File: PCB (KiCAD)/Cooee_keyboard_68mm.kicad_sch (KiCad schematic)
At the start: 99 parts, among them J1 Conn_01x15_Pin

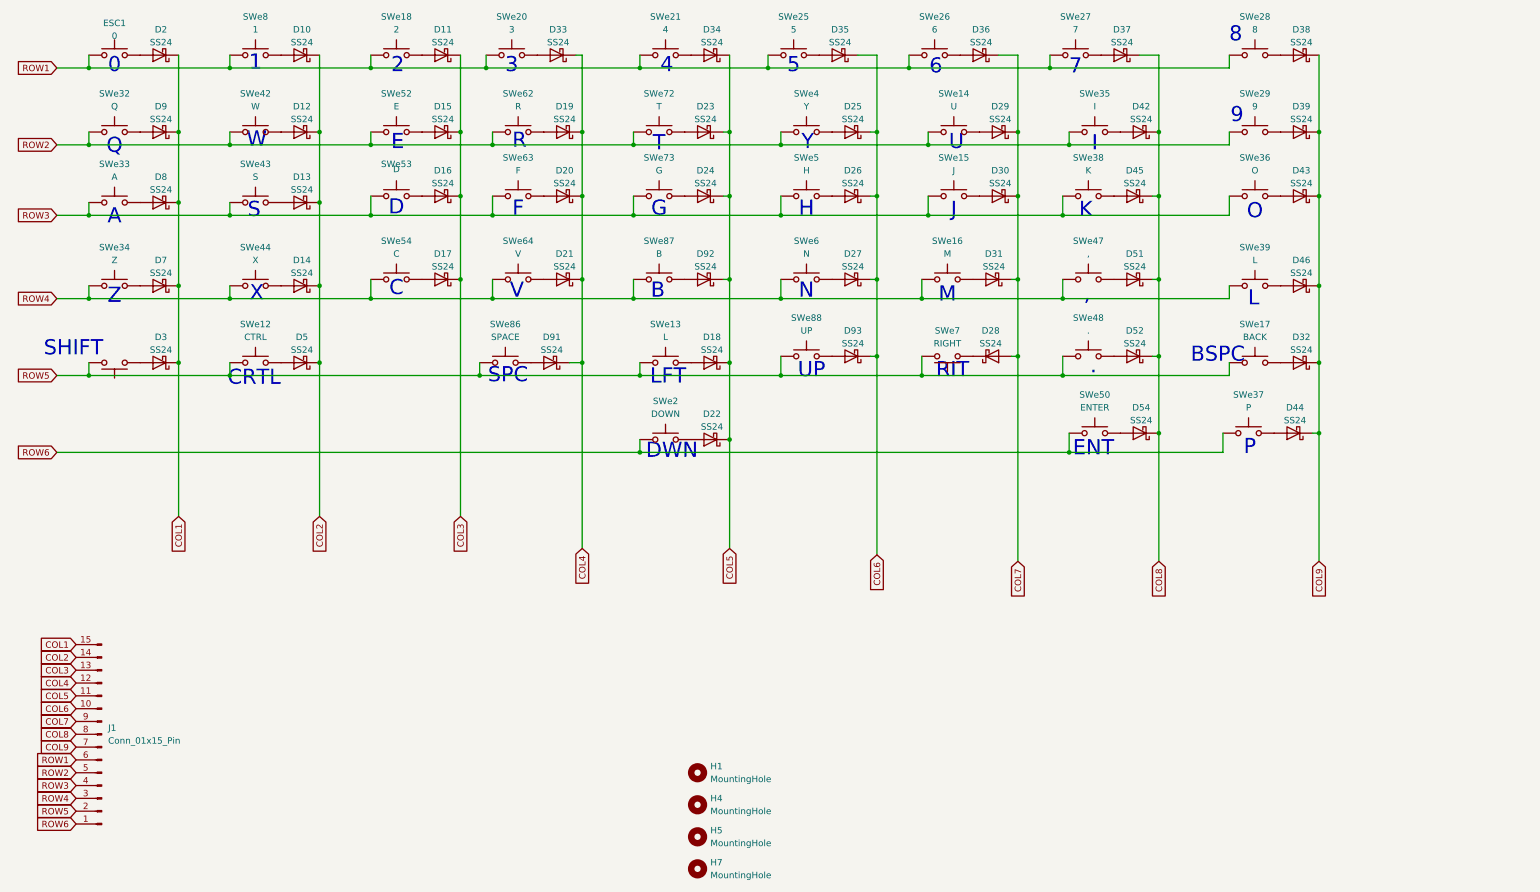
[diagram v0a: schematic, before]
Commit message: finished routing new smaller keyboard
finished routing new smaller keyboard
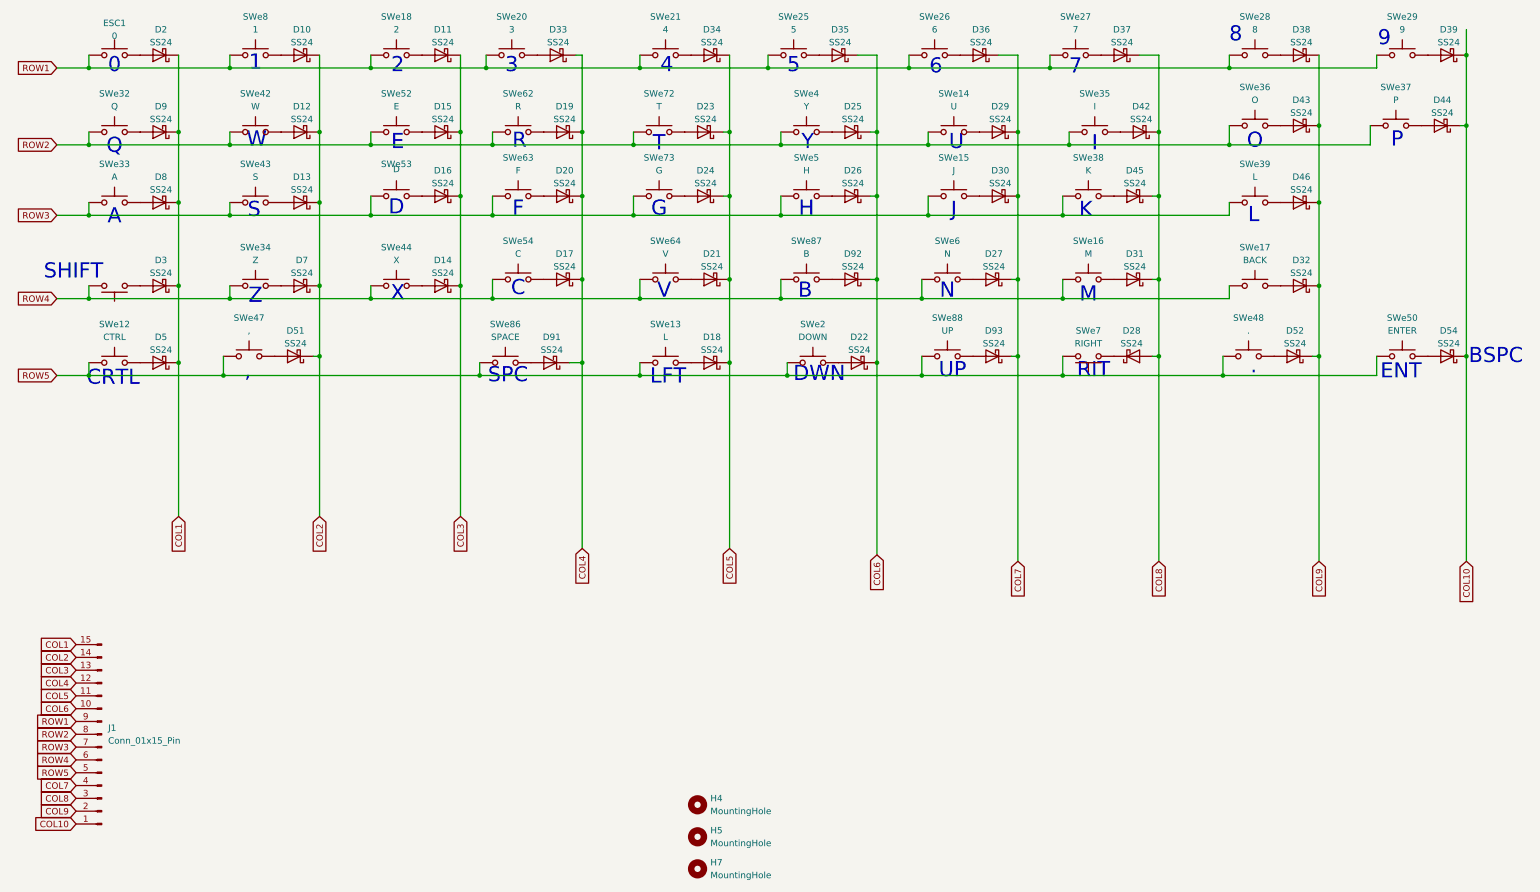
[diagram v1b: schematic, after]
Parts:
- removed H1: MountingHole, MountingHole:MountingHole_3.2mm_M3_ISO7380_Pad, symbol Mechanical:MountingHole
- H4, H5: footprint MountingHole:MountingHole_3.2mm_M3_ISO7380_Pad -> MountingHole:MountingHole_3.2mm_M3
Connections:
- net COL1: now also D5.1 (K); no longer D7.1 (K)
- net COL2: now also D51.1 (K), D7.1 (K); no longer D14.1 (K), D5.1 (K)
- net COL3: now also D14.1 (K); no longer D17.1 (K)
- net COL4: now also D17.1 (K); no longer D21.1 (K)
- net COL5: now also D21.1 (K); no longer D22.1 (K), D92.1 (K)
- net COL6: now also D22.1 (K), D92.1 (K); no longer D27.1 (K), D93.1 (K)
- net COL7: now also D27.1 (K), D93.1 (K), J1.4 (Pin_4); no longer D28.2 (A), D31.1 (K), J1.9 (Pin_9)
- net COL8: now also D28.2 (A), D31.1 (K), J1.3 (Pin_3); no longer D51.1 (K), D52.1 (K), D54.1 (K), J1.8 (Pin_8)
- net COL9: now also D52.1 (K), J1.2 (Pin_2); no longer D39.1 (K), D44.1 (K), J1.7 (Pin_7)
- net ROW1: now also J1.9 (Pin_9), SWe29.1; no longer J1.6 (Pin_6)
- net ROW2: now also J1.8 (Pin_8), SWe36.1, SWe37.1; no longer J1.5 (Pin_5), SWe29.1
- net ROW3: now also J1.7 (Pin_7), SWe39.1; no longer J1.4 (Pin_4), SWe36.1
- net ROW4: now also J1.6 (Pin_6), SWe17.1, SWe24.1; no longer J1.3 (Pin_3), SWe39.1, SWe47.1
- net ROW5: now also J1.5 (Pin_5), SWe2.1, SWe47.1, SWe50.1; no longer J1.2 (Pin_2), SWe17.1, SWe24.1
- removed net ROW6: J1.1 (Pin_1), SWe2.1, SWe37.1, SWe50.1
- new net COL10: D39.1 (K), D44.1 (K), D54.1 (K), J1.1 (Pin_1)
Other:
- moved on the sheet: D14, D17, D21, D22, D27, D28, D3, D31, D32, D39, D43, D44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
